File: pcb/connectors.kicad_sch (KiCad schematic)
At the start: 3 parts, among them J1 OBD2, J2 CAN, J3 TC2030

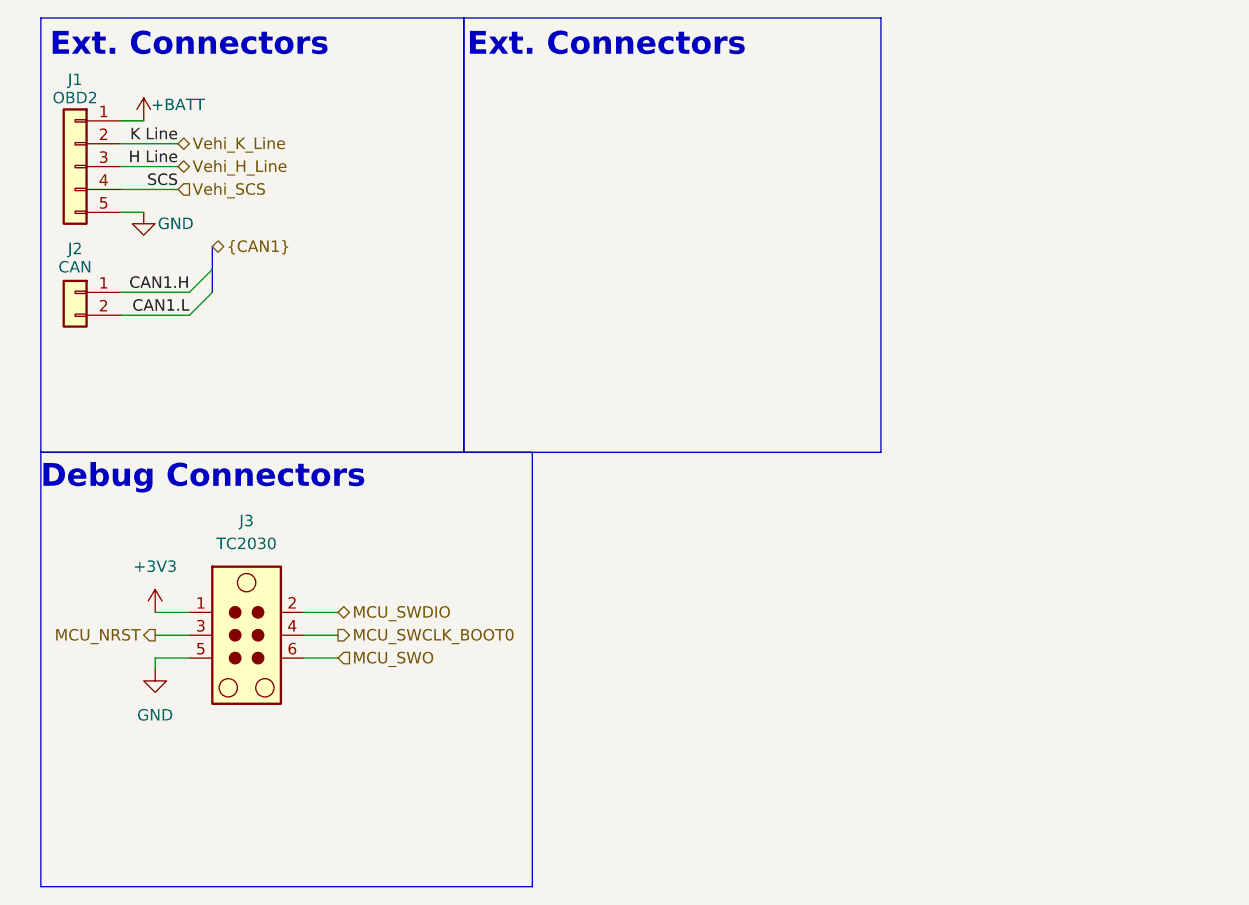
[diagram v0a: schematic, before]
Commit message: busses are hard
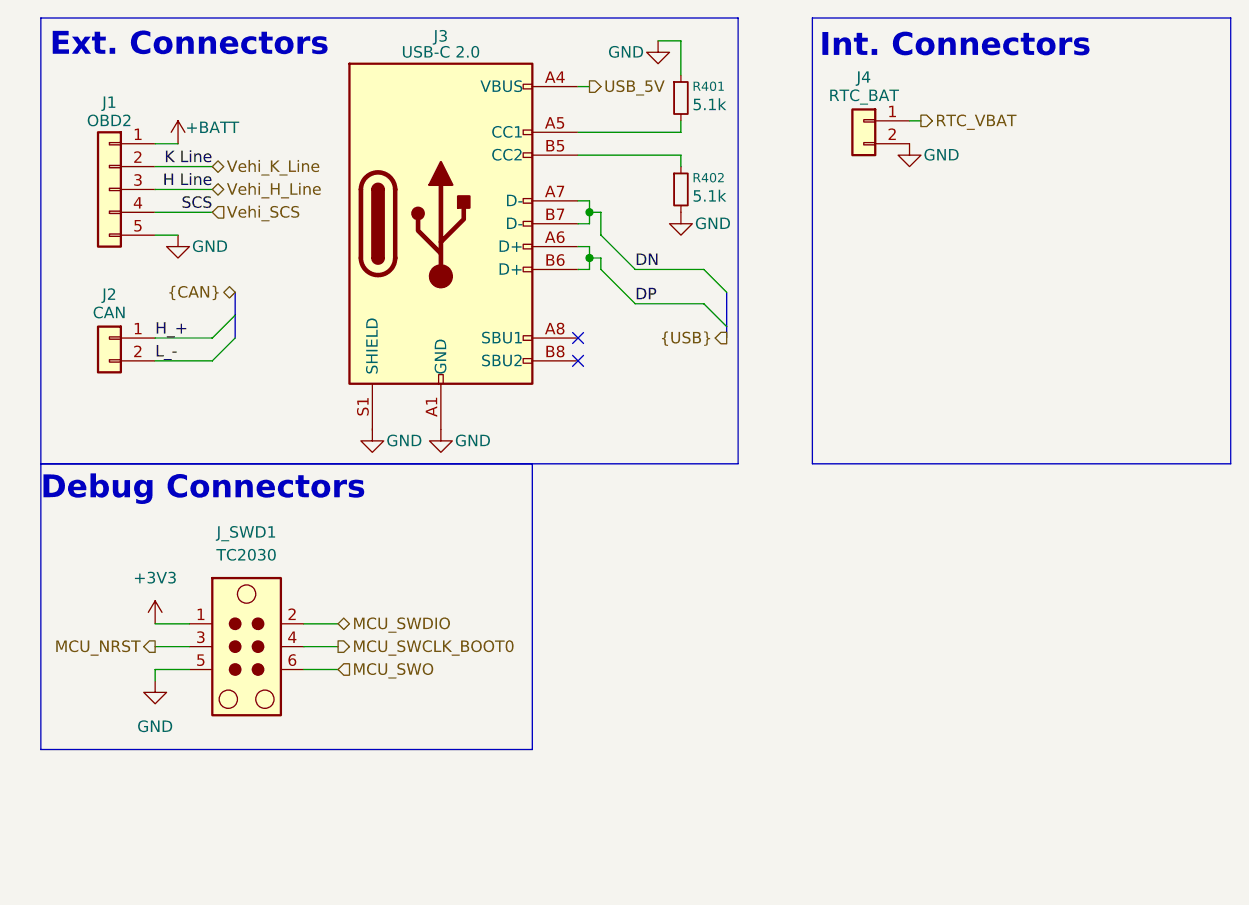
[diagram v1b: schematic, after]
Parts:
- added J3: USB-C 2.0, Connector_USB:USB_C_Receptacle_GCT_USB4105-xx-A_16P_TopMnt_Horizontal, symbol Connector:USB_C_Receptacle_USB2.0_16P
- added J4: RTC_BAT, Connector_Molex:Molex_PicoBlade_53047-0210_1x02_P1.25mm_Vertical, symbol Connector_Generic:Conn_01x02
- added R401, R402: 5.1k, Resistor_SMD:R_0402_1005Metric, symbol Device:R_Small
- renumbered J3 to J_SWD1
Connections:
- net GND: now also J3.A1 (GND), J3.A12 (GND), J3.B1 (GND), J3.B12 (GND), J3.S1 (SHIELD), J4.2 (Pin_2), R401.1, R402.2
- net CAN1.H renamed H_+
- net CAN1.L renamed L_-
- new net: J3.B5 (CC2), R402.1
- new net: J3.A5 (CC1), R401.2
- new net DN: J3.A7 (D-), J3.B7 (D-)
- new net DP: J3.A6 (D+), J3.B6 (D+)
- new net RTC_VBAT: J4.1 (Pin_1)
- new net USB_5V: J3.A4 (VBUS), J3.A9 (VBUS), J3.B4 (VBUS), J3.B9 (VBUS)
- no-connect marks 0 -> 2
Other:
- note added: "Int. Connectors"
- moved on the sheet: J1, J2, J_SWD1
